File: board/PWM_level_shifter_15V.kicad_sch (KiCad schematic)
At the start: 61 parts, among them J10 Conn_02x07_Odd_Even, J2 Conn_01x02_Pin, J3 Conn_01x02_Pin, J4 Conn_01x02_Pin, J5 Conn_01x02_Pin, J6 Conn_01x02_Pin, J7 Conn_01x02_Pin, J8 Conn_02x07_Odd_Even, J9 Conn_02x07_Odd_Even, U1 H11L1, U11 H11L1, U12 H11L1, U13 4049, U14 4049, U15 H11L1, U16 4049, U2 4049, U3 H11L1, U4 H11L1, U5 4049, U6 4049, U7 H11L1, U8 H11L1, U9 H11L1

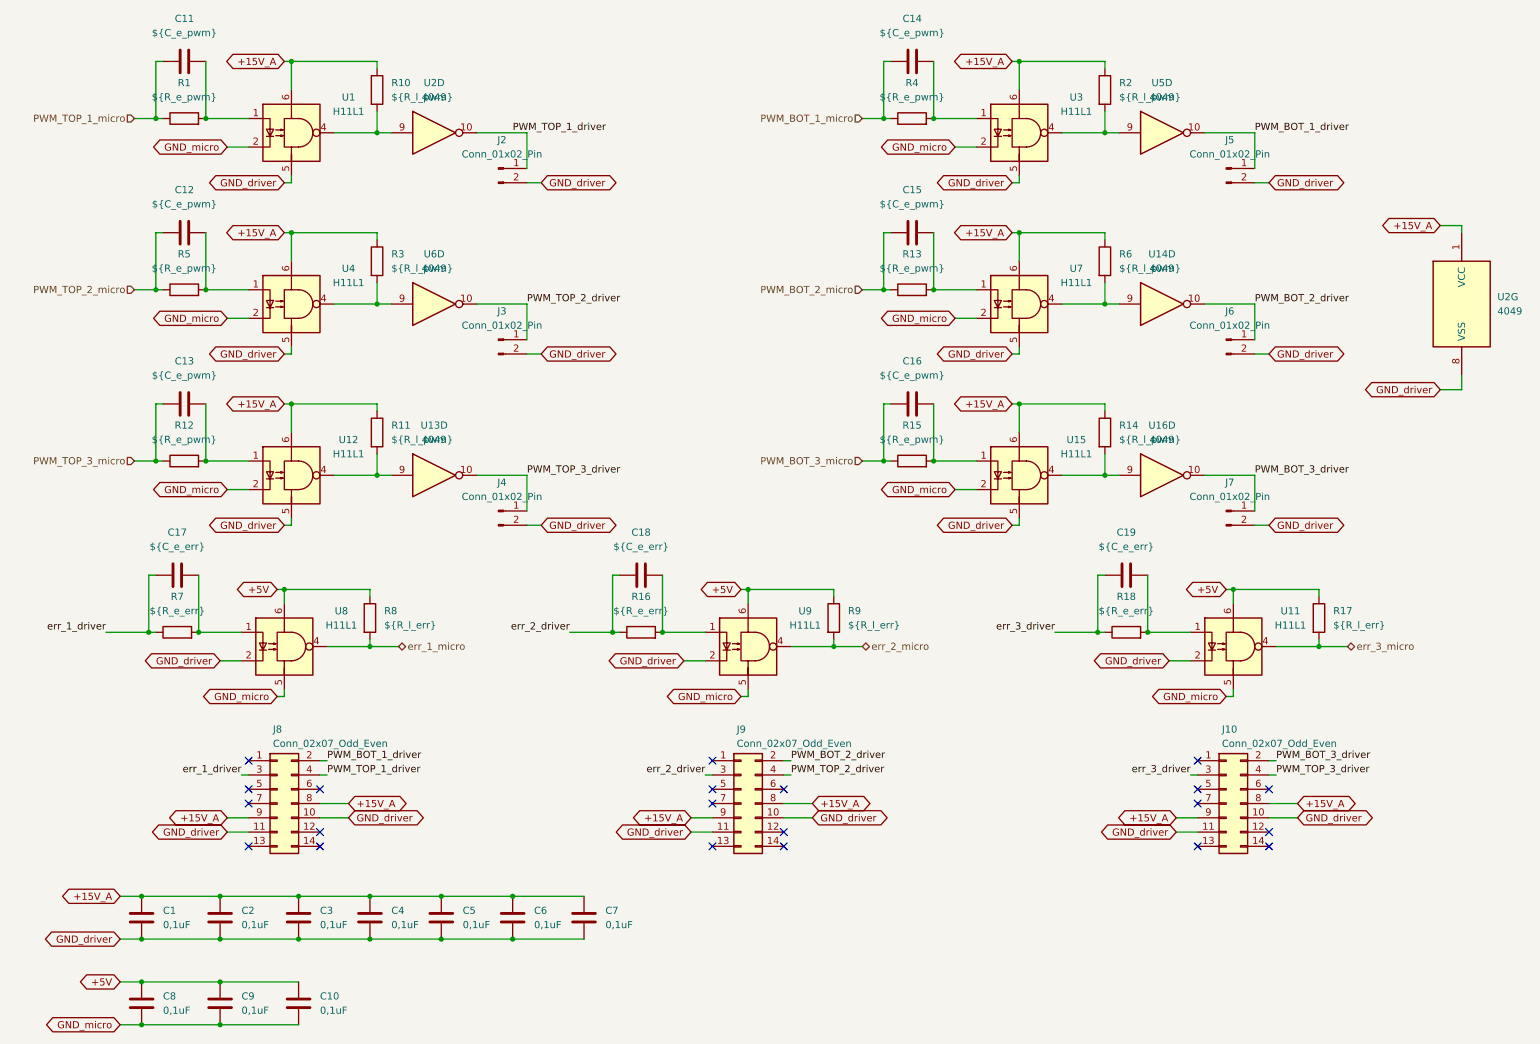
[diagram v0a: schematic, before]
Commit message: Schematic changes and board creation
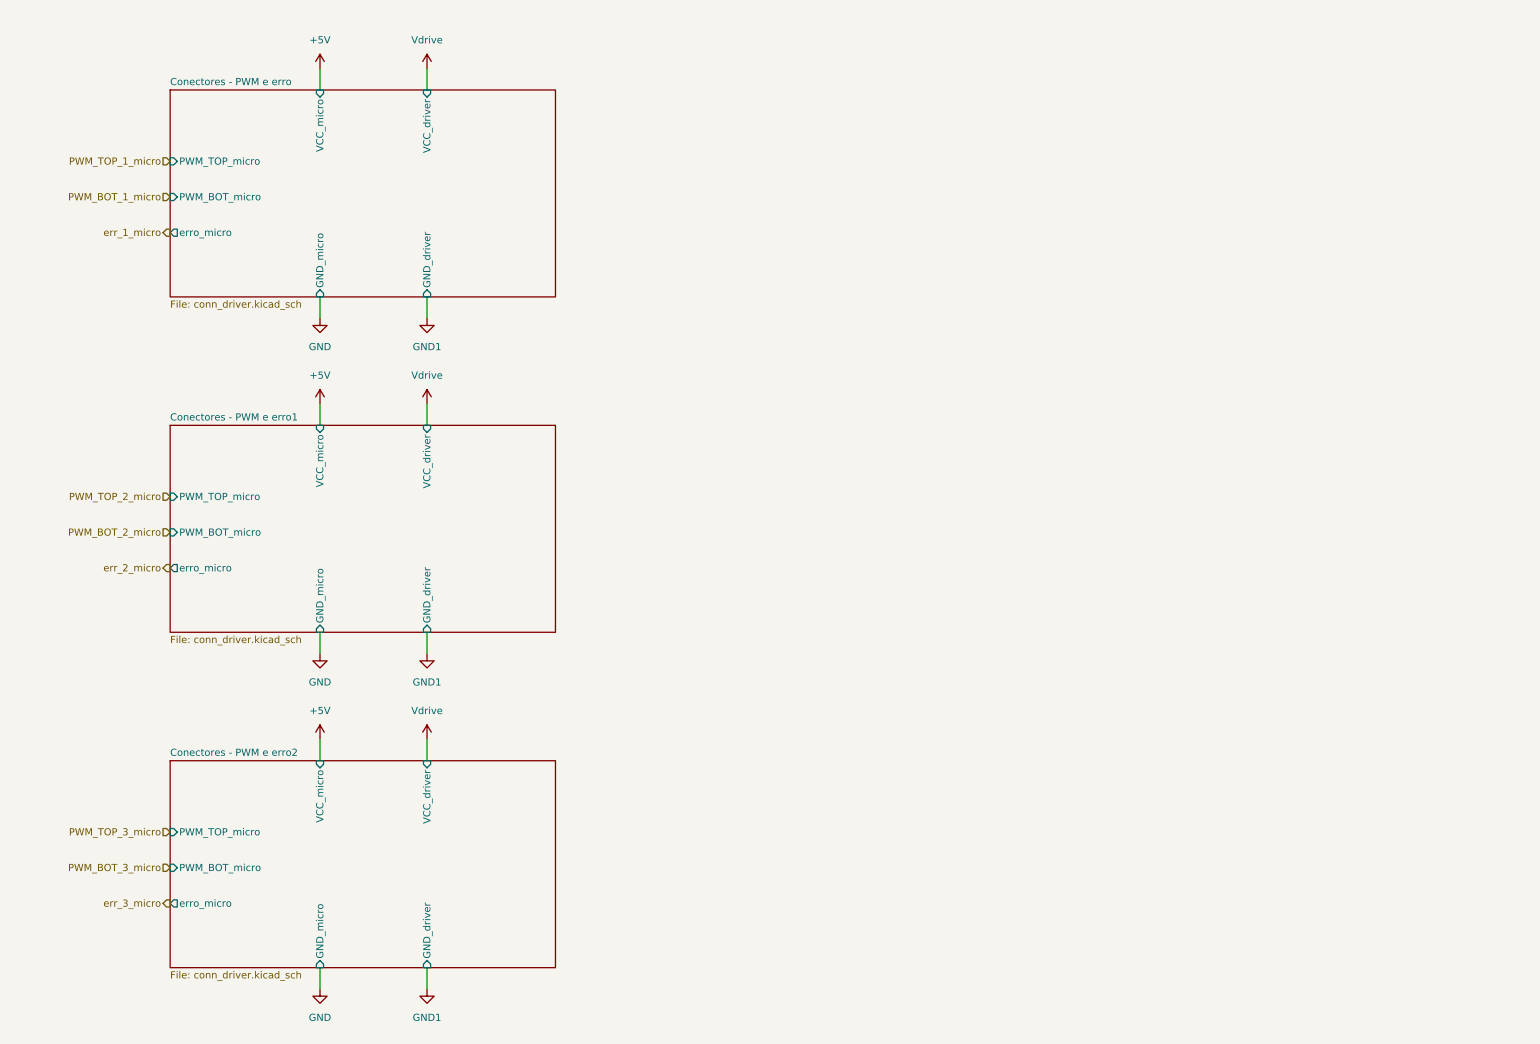
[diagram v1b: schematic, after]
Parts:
- removed C1, C10, C2, C3, C4, C5, C6, C7, C8, C9: 0,1uF, symbol Device:C
- removed C11, C12, C13, C14, C15, C16: ${C_e_pwm}, symbol Device:C
- removed C17, C18, C19: ${C_e_err}, symbol Device:C
- removed J10, J8, J9: Conn_02x07_Odd_Even, symbol Connector_Generic:Conn_02x07_Odd_Even
- removed J2, J3, J4, J5, J6, J7: Conn_01x02_Pin, symbol Connector:Conn_01x02_Pin
- removed R1, R12, R13, R15, R4, R5: ${R_e_pwm}, symbol Device:R
- removed R10, R11, R14, R2, R3, R6: ${R_l_pwm}, symbol Device:R
- removed R16, R18, R7: ${R_e_err}, symbol Device:R
- removed R17, R8, R9: ${R_l_err}, symbol Device:R
- removed U1, U11, U12, U15, U3, U4, U7, U8, U9: H11L1, symbol Isolator:H11L1
- removed U13, U14, U16, U2, U5, U6: 4049, symbol 4xxx:4049
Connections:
- no-connect marks 21 -> 0
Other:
- added sheet Conectores - PWM e erro (conn_driver.kicad_sch)
- added sheet Conectores - PWM e erro1 (conn_driver.kicad_sch)
- added sheet Conectores - PWM e erro2 (conn_driver.kicad_sch)
